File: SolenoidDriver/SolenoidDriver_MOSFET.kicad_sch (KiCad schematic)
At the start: 28 parts, among them Q1 Q_Dual_NMOS, Q2 Q_Dual_NMOS, Q3 Q_Dual_NMOS, Q4 Q_Dual_NMOS

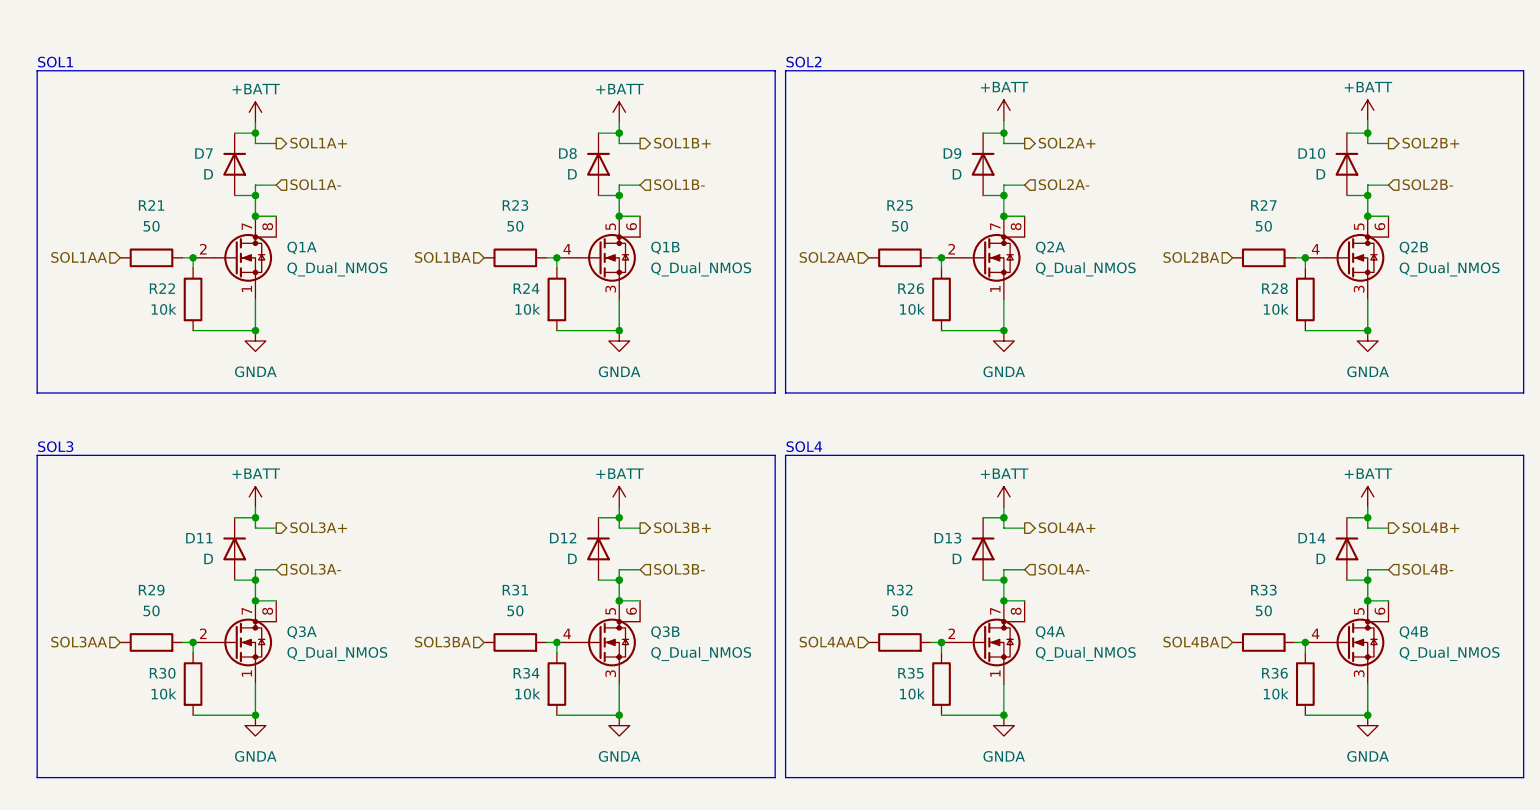
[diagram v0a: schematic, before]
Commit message: Solenoid Driver ver1.1
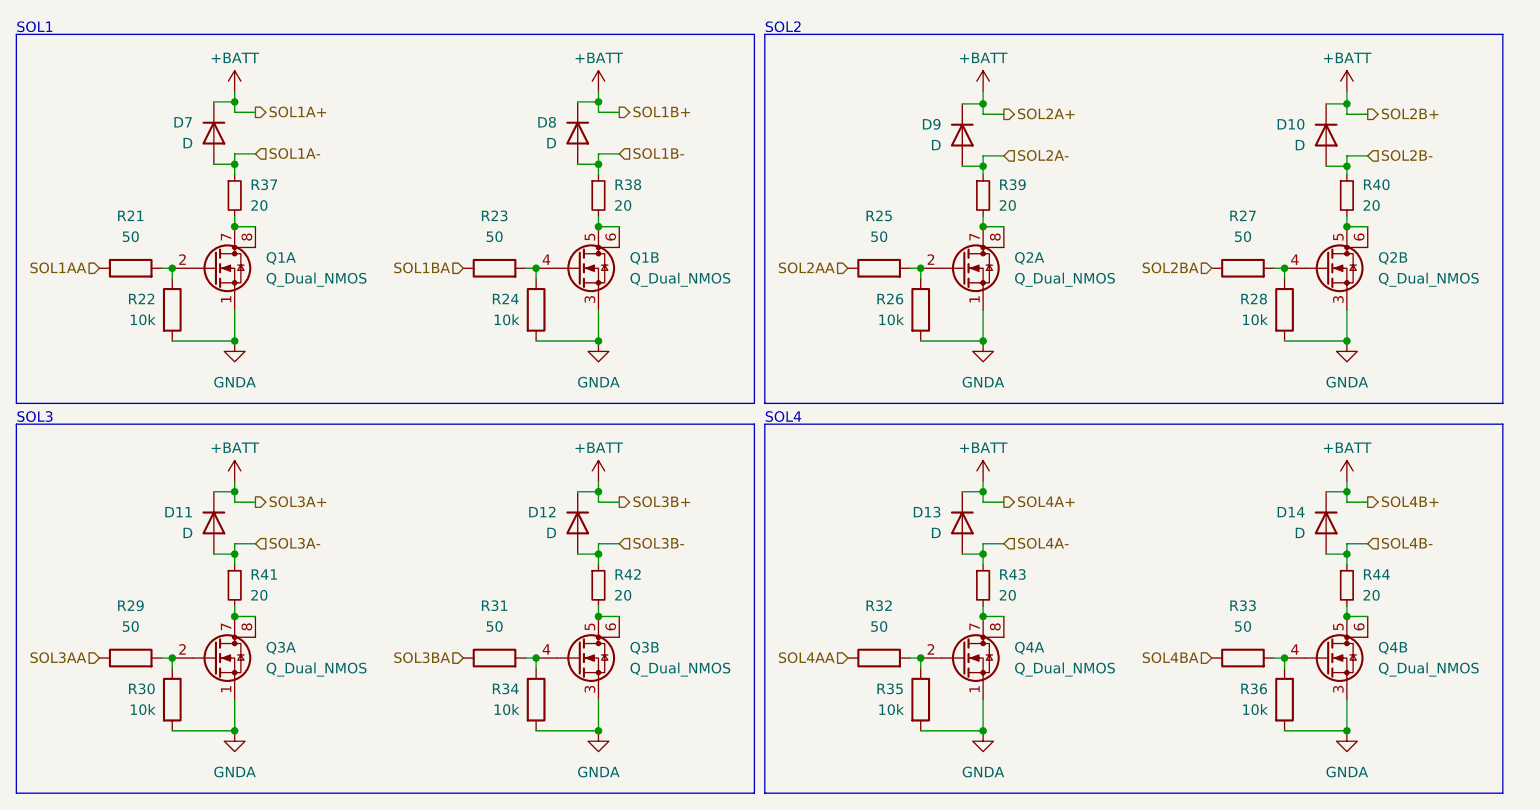
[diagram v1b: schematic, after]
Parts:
- added R37, R38, R39, R40, R41, R42, R43, R44: 20, Resistor_SMD:R_0603_1608Metric, symbol Device:R_Small
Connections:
- net SOL1A-: now also R37.1; no longer Q1.7 (D), Q1.8 (D)
- net SOL1B-: now also R38.1; no longer Q1.5 (D), Q1.6 (D)
- net SOL2A-: now also R39.1; no longer Q2.7 (D), Q2.8 (D)
- net SOL2B-: now also R40.1; no longer Q2.5 (D), Q2.6 (D)
- net SOL3A-: now also R41.1; no longer Q3.7 (D), Q3.8 (D)
- net SOL3B-: now also R42.1; no longer Q3.5 (D), Q3.6 (D)
- net SOL4A-: now also R43.1; no longer Q4.7 (D), Q4.8 (D)
- net SOL4B-: now also R44.1; no longer Q4.5 (D), Q4.6 (D)
- new net: Q2.7 (D), Q2.8 (D), R39.2
- new net: Q1.5 (D), Q1.6 (D), R38.2
- new net: Q2.5 (D), Q2.6 (D), R40.2
- new net: Q4.7 (D), Q4.8 (D), R43.2
- new net: Q1.7 (D), Q1.8 (D), R37.2
- new net: Q3.7 (D), Q3.8 (D), R41.2
- new net: Q4.5 (D), Q4.6 (D), R44.2
- new net: Q3.5 (D), Q3.6 (D), R42.2
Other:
- moved on the sheet: D10, D11, D12, D13, D14, D7, D8, D9, Q1A, Q1B, Q2A, Q2B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
